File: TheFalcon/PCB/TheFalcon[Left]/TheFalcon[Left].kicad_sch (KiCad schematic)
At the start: 42 parts, among them J2 Conn_01x04_Pin, J3 Conn_01x04_Pin, J5 Conn_01x01, J6 Conn_01x01, SW1 SW_Push, SW2 SW_Push, U2 USBLC6-2P6, U3 USBLC6-2P6, U4 AMS1117-3.3, U6 STM32G431CBTx, Y1 X322516MOB4SI

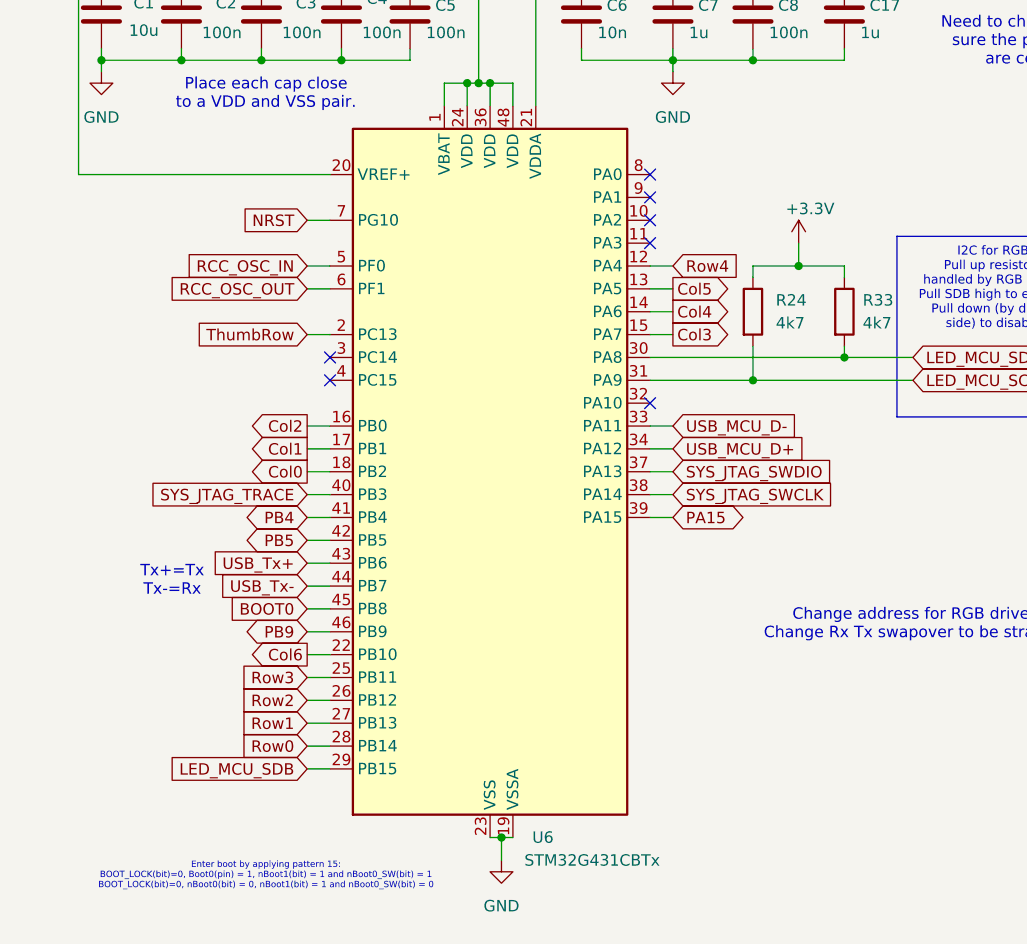
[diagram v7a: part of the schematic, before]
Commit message: Save
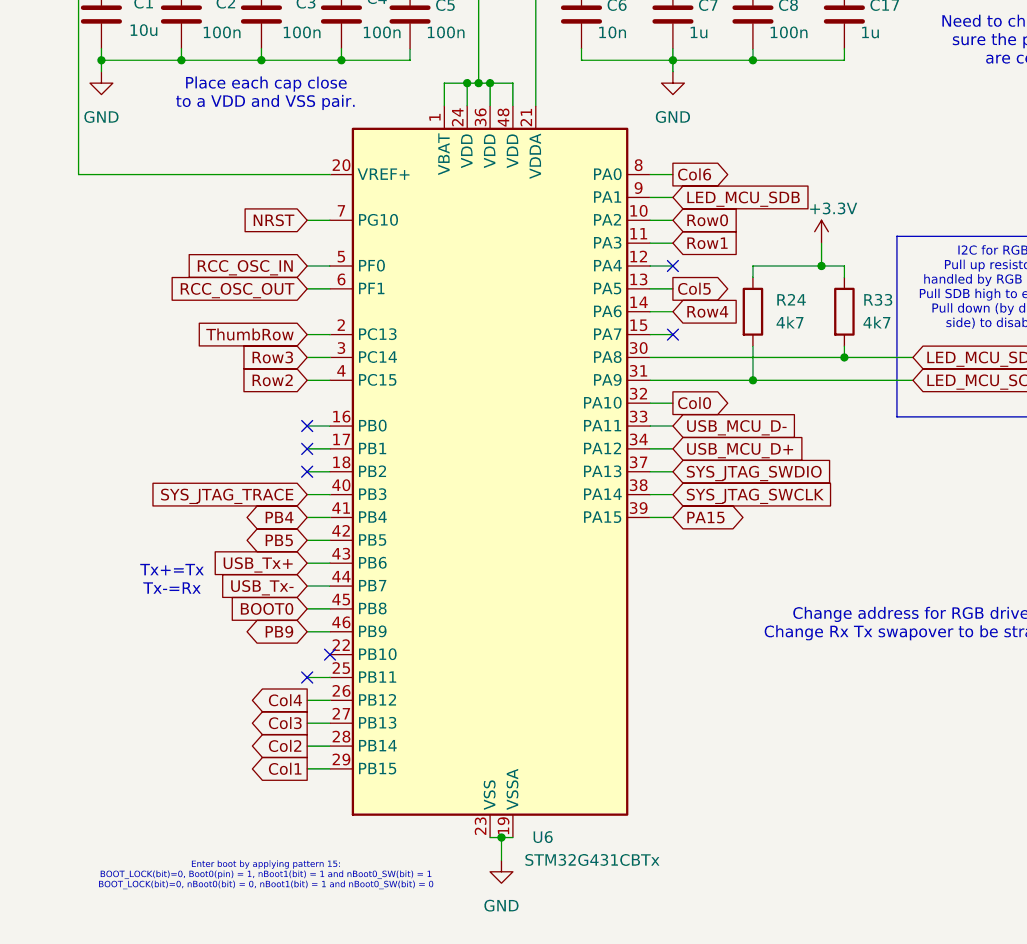
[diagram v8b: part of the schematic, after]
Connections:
- net Col0: now also U6.32 (PA10); no longer U6.18 (PB2)
- net Col1: now also U6.29 (PB15); no longer U6.17 (PB1)
- net Col2: now also U6.28 (PB14); no longer U6.16 (PB0)
- net Col3: now also U6.27 (PB13); no longer U6.15 (PA7)
- net Col4: now also U6.26 (PB12); no longer U6.14 (PA6)
- net Col6: now also U6.8 (PA0); no longer U6.22 (PB10)
- net LED_MCU_SDB: now also U6.9 (PA1); no longer U6.29 (PB15)
- net Row0: now also U6.10 (PA2); no longer U6.28 (PB14)
- net Row1: now also U6.11 (PA3); no longer U6.27 (PB13)
- net Row2: now also U6.4 (PC15); no longer U6.26 (PB12)
- net Row3: now also U6.3 (PC14); no longer U6.25 (PB11)
- net Row4: now also U6.14 (PA6); no longer U6.12 (PA4)
